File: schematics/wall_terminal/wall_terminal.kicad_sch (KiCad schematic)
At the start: 21 parts, among them J1 6P6C, J2 6P6C, J3 Conn_02x12_Odd_Even, Q1 2N7000, U1 ATtiny13A-P, U2 MAX487E

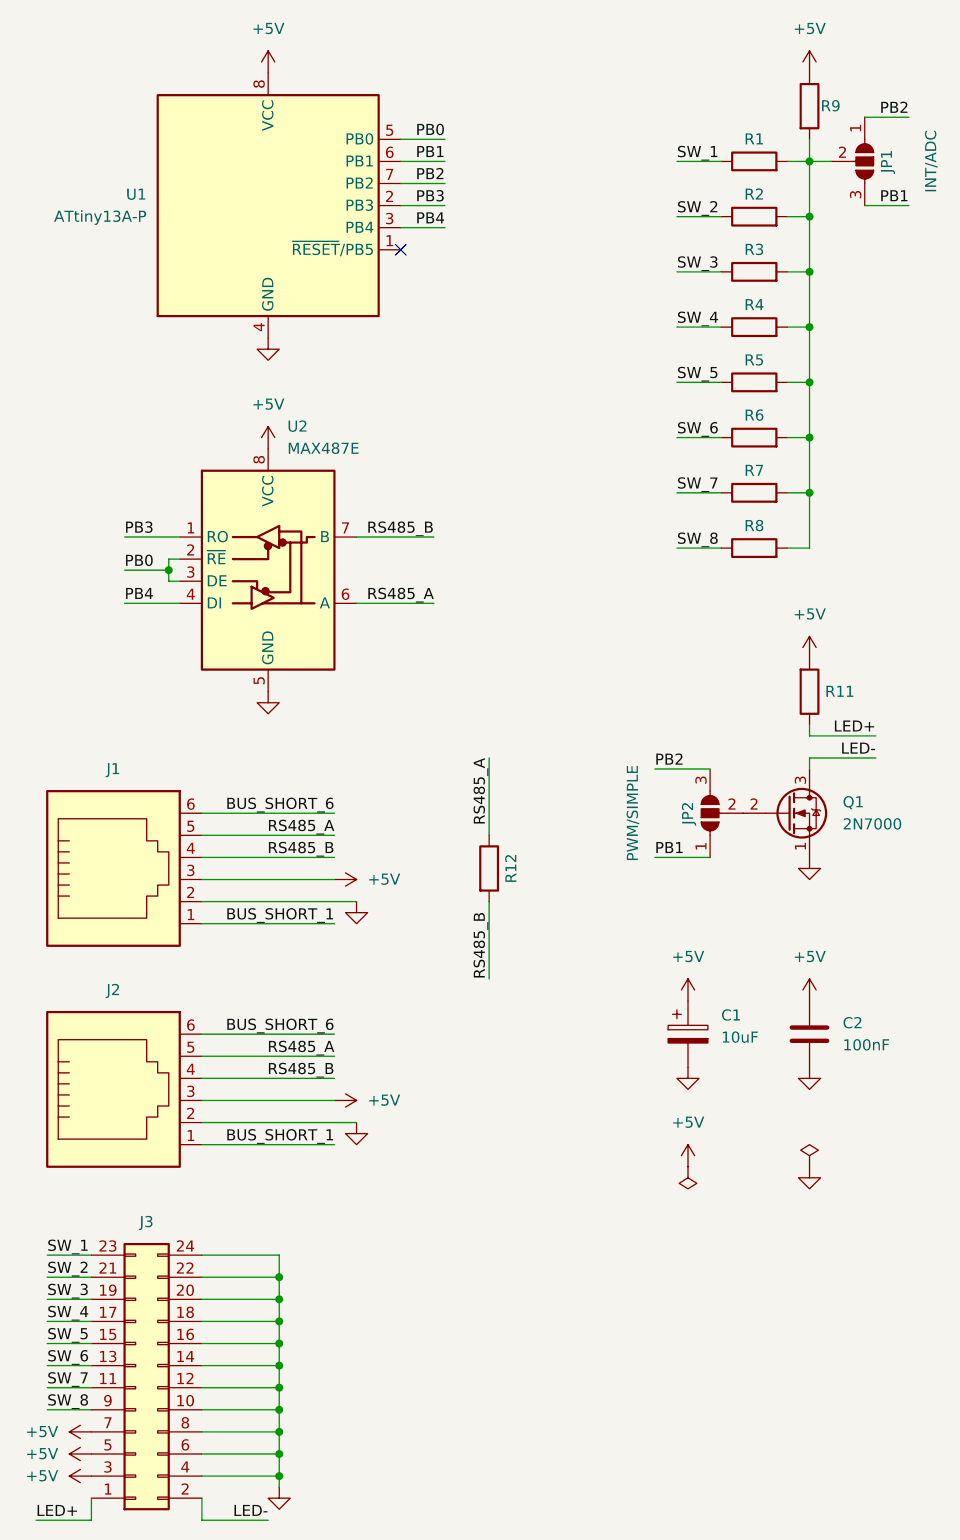
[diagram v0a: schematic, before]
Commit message: !feat: first wall terminal PCB prototype.
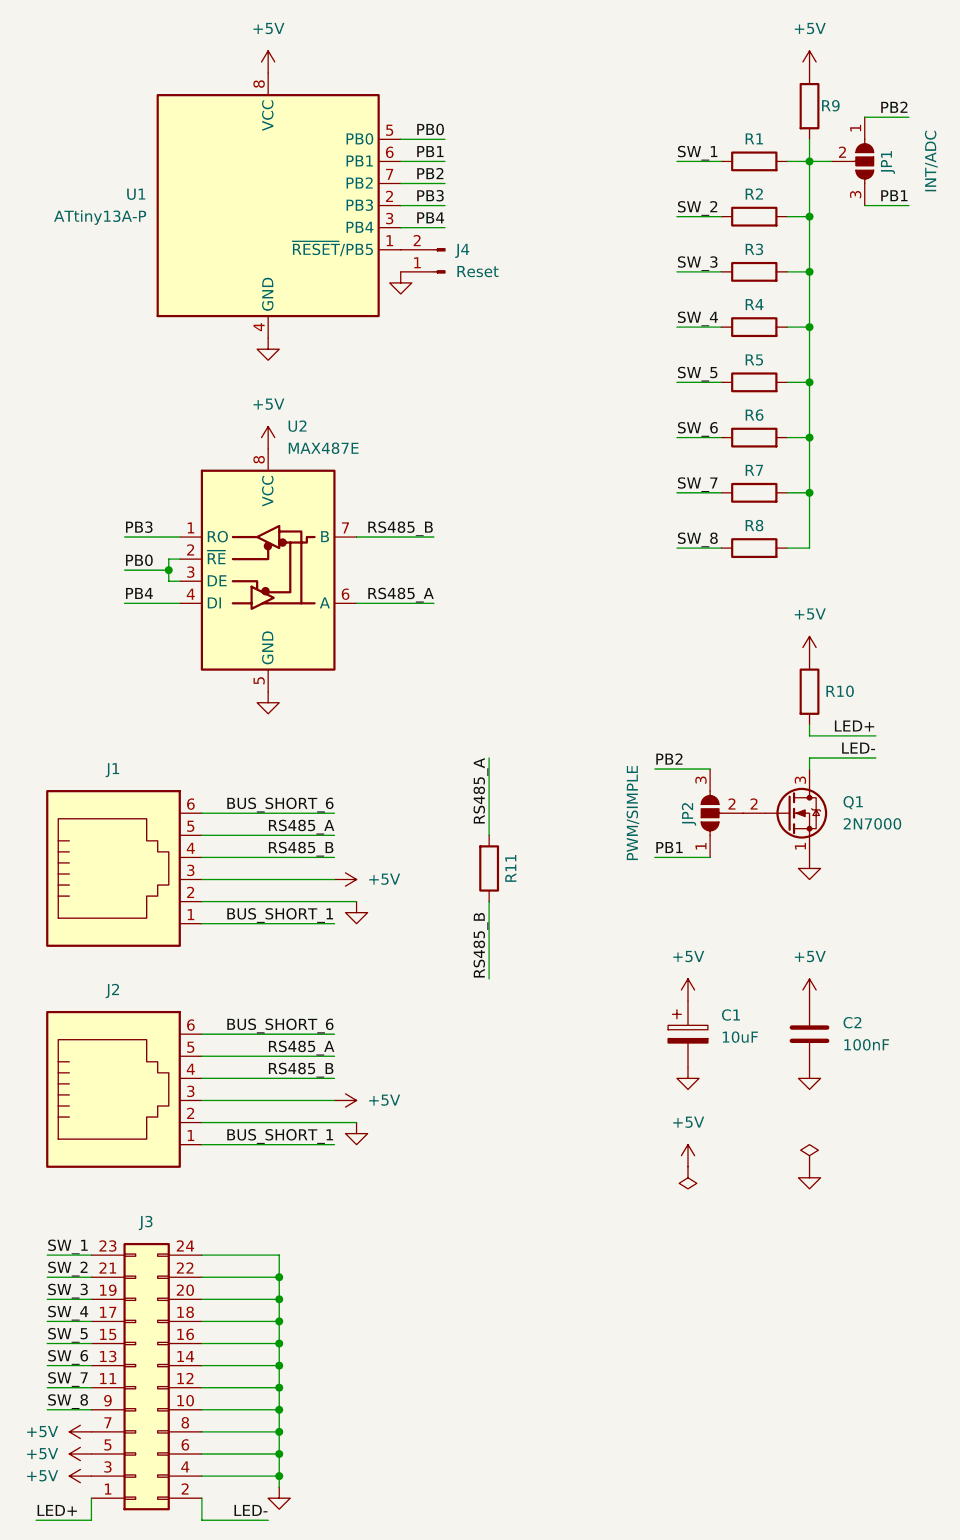
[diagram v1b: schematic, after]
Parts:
- added J4: Reset, Connector_PinHeader_2.54mm:PinHeader_1x02_P2.54mm_Vertical, symbol Connector:Conn_01x02_Pin
- renumbered R11 to R10, R12 to R11
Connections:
- net +5V: now also R10.1; no longer R10.2
- net GND: now also J4.1 (Pin_1)
- net LED+: now also R10.2; no longer R10.1
- net RS485_A: now also R11.2; no longer R11.1
- net RS485_B: now also R11.1; no longer R11.2
- net at U1.1 (~{RESET}/PB5): now also J4.2 (Pin_2)
- no-connect marks 1 -> 0
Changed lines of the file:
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@@
 		(color 0 0 0 0)
 	)
-	(no_connect
-		(at 60.96 45.72)
-	)
 	(wire
 		(pts
@@
 		(lib_id "Device:R")
 		(at 107.95 96.52 0)
-		(mirror x)
 		(unit 1)
 		(exclude_from_sim no)
@@
 		(on_board yes)
 		(dnp no)
-		(property "Reference" "R11"
+		(property "Reference" "R10"
 			(at 109.728 96.52 0)
 			(effects
@@
 		)
 		(property "Value" "R"
-			(at 110.49 95.2501 0)
+			(at 110.49 97.7899 0)
 			(effects
 				(font
@@
 			(project "wall_terminal"
 				(path "/5c441dea-07fa-47c6-a7dc-b1c524c62a23"
-					(reference "R11")
+					(reference "R10")
 					(unit 1)
 				)
@@
 		(lib_id "Device:R")
 		(at 71.12 116.84 0)
+		(mirror x)
 		(unit 1)
 		(exclude_from_sim no)
@@
 		(on_board yes)
 		(dnp no)
-		(property "Reference" "R12"
+		(property "Reference" "R11"
 			(at 73.66 116.84 90)
 			(effects
@@
 			(project "wall_terminal"
 				(path "/5c441dea-07fa-47c6-a7dc-b1c524c62a23"
-					(reference "R12")
+					(reference "R11")
 					(unit 1)
 				)
@@
 	)
 	(symbol
+		(lib_id "Connector:Conn_01x02_Pin")
+		(at 66.04 48.26 180)
+		(unit 1)
+		(exclude_from_sim no)
+		(in_bom yes)
+		(on_board yes)
+		(dnp no)
+		(fields_autoplaced yes)
+		(property "Reference" "J4"
+			(at 67.31 45.7199 0)
+			(effects
+				(font
+					(size 1.27 1.27)
+				)
+				(justify right)
+			)
+		)
+		(property "Value" "Reset"
+			(at 67.31 48.2599 0)
+			(effects
+				(font
+					(size 1.27 1.27)
+				)
+				(justify right)
+			)
+		)
+		(property "Footprint" "Connector_PinHeader_2.54mm:PinHeader_1x02_P2.54mm_Vertical"
+			(at 66.04 48.26 0)
+			(effects
+				(font
+					(size 1.27 1.27)
+				)
+				(hide yes)
+			)
+		)
+		(property "Datasheet" "~"
+			(at 66.04 48.26 0)
+			(effects
+				(font
+					(size 1.27 1.27)
+				)
+				(hide yes)
+			)
+		)
+		(property "Description" "Generic connector, single row, 01x02, script generated"
+			(at 66.04 48.26 0)
+			(effects
+				(font
+					(size 1.27 1.27)
+				)
+				(hide yes)
+			)
+		)
+		(pin "1"
+		)
+		(pin "2"
+		)
+		(instances
+			(project "wall_terminal"
+				(path "/5c441dea-07fa-47c6-a7dc-b1c524c62a23"
+					(reference "J4")
+					(unit 1)
+				)
+			)
+		)
+	)
+	(symbol
 		(lib_id "power:GND")
 		(at 45.72 96.52 0)
@@
 					(unit 1)
 				)
+			)
+		)
+	)
+	(symbol
+		(lib_id "power:GND")
+		(at 60.96 48.26 0)
+		(unit 1)
+		(exclude_from_sim no)
+		(in_bom yes)
+		(on_board yes)
+		(dnp no)
+		(fields_autoplaced yes)
+		(property "Reference" "#PWR09"
+			(at 60.96 54.61 0)
+			(effects
+				(font
+					(size 1.27 1.27)
+				)
+				(hide yes)
+			)
+		)
+		(property "Value" "GND"
+			(at 60.96 53.34 0)
+			(effects
+				(font
+					(size 1.27 1.27)
+				)
+				(hide yes)
+			)
+		)
+		(property "Footprint" ""
+			(at 60.96 48.26 0)
+			(effects
+				(font
+					(size 1.27 1.27)
+				)
+				(hide yes)
+			)
+		)
+		(property "Datasheet" ""
+			(at 60.96 48.26 0)
+			(effects
+				(font
+					(size 1.27 1.27)
+				)
+				(hide yes)
+			)
+		)
+		(property "Description" "Power symbol creates a global label with name \"GND\" , ground"
+			(at 60.96 48.26 0)
+			(effects
+				(font
+					(size 1.27 1.27)
+				)
+				(hide yes)
+			)
+		)
+		(pin "1"
+		)
+		(instances
+			(project "wall_terminal"
+				(path "/5c441dea-07fa-47c6-a7dc-b1c524c62a23"
+					(reference "#PWR09")
+					(unit 1)
+				)
